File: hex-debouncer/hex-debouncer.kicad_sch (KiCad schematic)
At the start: 37 parts, among them J1 Conn_01x08, SW1 A, SW2 B, SW3 C, SW4 D, SW5 E, SW6 F, U1 74HC14

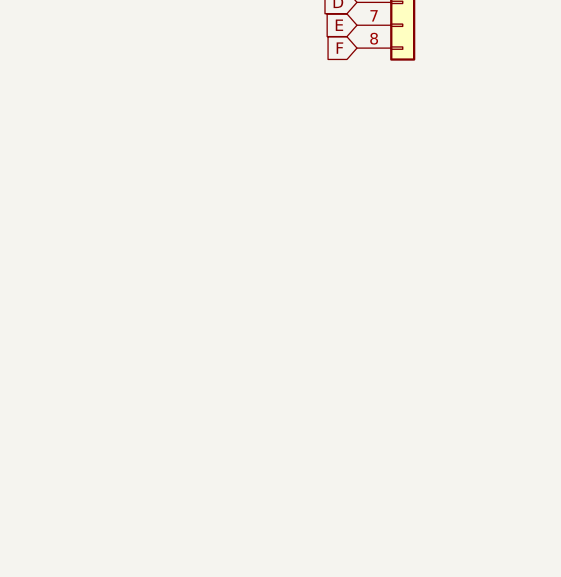
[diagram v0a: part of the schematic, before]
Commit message: up
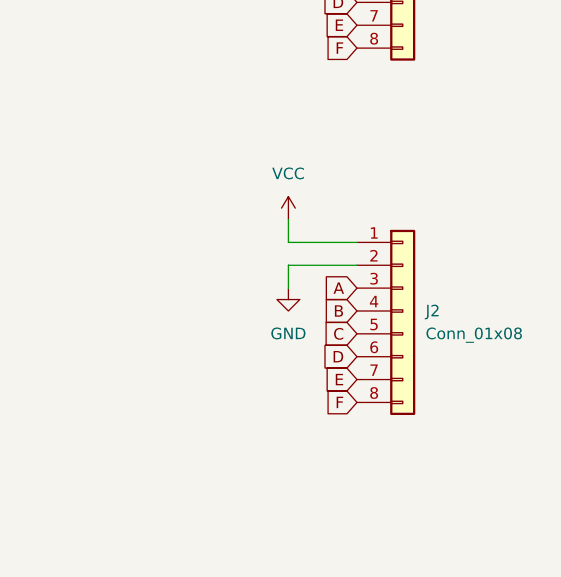
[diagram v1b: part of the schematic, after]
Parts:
- added J2: Conn_01x08, Connector_PinHeader_2.54mm:PinHeader_1x08_P2.54mm_Vertical, symbol Connector_Generic:Conn_01x08
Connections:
- net A: now also J2.3 (Pin_3)
- net B: now also J2.4 (Pin_4)
- net C: now also J2.5 (Pin_5)
- net D: now also J2.6 (Pin_6)
- net E: now also J2.7 (Pin_7)
- net F: now also J2.8 (Pin_8)
- net GND: now also J2.2 (Pin_2)
- net VCC: now also J2.1 (Pin_1)
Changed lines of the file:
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@@
+    (stroke (width 0) (type default) (color 0 0 0 0))
+  )
+  (wire (pts (xy 246.38 81.28) (xy 246.38 83.82))
     (stroke (width 0) (type default) (color 0 0 0 0))
   )
@@
     (stroke (width 0) (type default) (color 0 0 0 0))
   )
+  (wire (pts (xy 254 81.28) (xy 246.38 81.28))
+    (stroke (width 0) (type default) (color 0 0 0 0))
+  )
   (wire (pts (xy 107.95 43.18) (xy 107.95 45.72))
     (stroke (width 0) (type default) (color 0 0 0 0))
@@
     (stroke (width 0) (type default) (color 0 0 0 0))
   )
+  (wire (pts (xy 254 78.74) (xy 246.38 78.74))
+    (stroke (width 0) (type default) (color 0 0 0 0))
+  )
   (wire (pts (xy 64.77 43.18) (xy 64.77 45.72))
     (stroke (width 0) (type default) (color 0 0 0 0))
@@
   )
   (wire (pts (xy 123.19 38.1) (xy 123.19 43.18))
+    (stroke (width 0) (type default) (color 0 0 0 0))
+  )
+  (wire (pts (xy 246.38 76.2) (xy 246.38 78.74))
     (stroke (width 0) (type default) (color 0 0 0 0))
   )
@@
     )
   )
+  (global_label "D" (shape input) (at 254 91.44 180) (fields_autoplaced)
+    (effects (font (size 1.27 1.27)) (justify right))
+    (property "Intersheet References" "${INTERSHEET_REFS}" (id 0) (at 250.3169 91.5194 0)
+      (effects (font (size 1.27 1.27)) (justify right) hide)
+    )
+  )
   (global_label "D" (shape input) (at 254 52.07 180) (fields_autoplaced)
     (effects (font (size 1.27 1.27)) (justify right))
@@
     )
   )
+  (global_label "A" (shape input) (at 254 83.82 180) (fields_autoplaced)
+    (effects (font (size 1.27 1.27)) (justify right))
+    (property "Intersheet References" "${INTERSHEET_REFS}" (id 0) (at 250.4983 83.8994 0)
+      (effects (font (size 1.27 1.27)) (justify right) hide)
+    )
+  )
   (global_label "D" (shape input) (at 97.79 86.36 0) (fields_autoplaced)
     (effects (font (size 1.27 1.27)) (justify left))
@@
     )
   )
+  (global_label "C" (shape input) (at 254 88.9 180) (fields_autoplaced)
+    (effects (font (size 1.27 1.27)) (justify right))
+    (property "Intersheet References" "${INTERSHEET_REFS}" (id 0) (at 250.3169 88.9794 0)
+      (effects (font (size 1.27 1.27)) (justify right) hide)
+    )
+  )
   (global_label "F" (shape input) (at 254 57.15 180) (fields_autoplaced)
     (effects (font (size 1.27 1.27)) (justify right))
@@
     )
   )
+  (global_label "E" (shape input) (at 254 93.98 180) (fields_autoplaced)
+    (effects (font (size 1.27 1.27)) (justify right))
+    (property "Intersheet References" "${INTERSHEET_REFS}" (id 0) (at 250.4379 94.0594 0)
+      (effects (font (size 1.27 1.27)) (justify right) hide)
+    )
+  )
   (global_label "F" (shape input) (at 140.97 86.36 0) (fields_autoplaced)
     (effects (font (size 1.27 1.27)) (justify left))
     (property "Intersheet References" "${INTERSHEET_REFS}" (id 0) (at 144.4717 86.2806 0)
       (effects (font (size 1.27 1.27)) (justify left) hide)
+    )
+  )
+  (global_label "B" (shape input) (at 254 86.36 180) (fields_autoplaced)
+    (effects (font (size 1.27 1.27)) (justify right))
+    (property "Intersheet References" "${INTERSHEET_REFS}" (id 0) (at 250.3169 86.4394 0)
+      (effects (font (size 1.27 1.27)) (justify right) hide)
+    )
+  )
+  (global_label "F" (shape input) (at 254 96.52 180) (fields_autoplaced)
+    (effects (font (size 1.27 1.27)) (justify right))
+    (property "Intersheet References" "${INTERSHEET_REFS}" (id 0) (at 250.4983 96.5994 0)
+      (effects (font (size 1.27 1.27)) (justify right) hide)
     )
   )
@@
     (pin "7")
   )
+  (symbol (lib_id "power:VCC") (at 246.38 76.2 0) (unit 1)
+    (in_bom yes) (on_board yes) (fields_autoplaced)
+    (property "Reference" "#PWR028" (id 0) (at 246.38 80.01 0)
+      (effects (font (size 1.27 1.27)) hide)
+    )
+    (property "Value" "VCC" (id 1) (at 246.38 71.12 0))
+    (property "Footprint" "" (id 2) (at 246.38 76.2 0)
+      (effects (font (size 1.27 1.27)) hide)
+    )
+    (property "Datasheet" "" (id 3) (at 246.38 76.2 0)
+      (effects (font (size 1.27 1.27)) hide)
+    )
+    (pin "1")
+  )
   (symbol (lib_id "Diode:LL4148") (at 30.48 86.36 180) (unit 1)
     (in_bom yes) (on_board yes) (fields_autoplaced)
@@
     (pin "1")
     (pin "2")
+  )
+  (symbol (lib_id "power:GND") (at 246.38 83.82 0) (unit 1)
+    (in_bom yes) (on_board yes)
+    (property "Reference" "#PWR029" (id 0) (at 246.38 90.17 0)
+      (effects (font (size 1.27 1.27)) hide)
+    )
+    (property "Value" "GND" (id 1) (at 246.38 88.9 0))
+    (property "Footprint" "" (id 2) (at 246.38 83.82 0)
+      (effects (font (size 1.27 1.27)) hide)
+    )
+    (property "Datasheet" "" (id 3) (at 246.38 83.82 0)
+      (effects (font (size 1.27 1.27)) hide)
+    )
+    (pin "1")
   )
   (symbol (lib_id "74xx:74HC14") (at 46.99 86.36 0) (unit 2)
@@
     (pin "1")
   )
+  (symbol (lib_id "Connector_Generic:Conn_01x08") (at 259.08 86.36 0) (unit 1)
+    (in_bom yes) (on_board yes) (fields_autoplaced)
+    (property "Reference" "J2" (id 0) (at 261.62 86.3599 0)
+      (effects (font (size 1.27 1.27)) (justify left))
+    )
+    (property "Value" "Conn_01x08" (id 1) (at 261.62 88.8999 0)
+      (effects (font (size 1.27 1.27)) (justify left))
+    )
+    (property "Footprint" "Connector_PinHeader_2.54mm:PinHeader_1x08_P2.54mm_Vertical" (id 2) (at 259.08 86.36 0)
+      (effects (font (size 1.27 1.27)) hide)
+    )
+    (property "Datasheet" "~" (id 3) (at 259.08 86.36 0)
+      (effects (font (size 1.27 1.27)) hide)
+    )
+    (pin "1")
+    (pin "2")
+    (pin "3")
+    (pin "4")
+    (pin "5")
+    (pin "6")
+    (pin "7")
+    (pin "8")
+  )
   (symbol (lib_id "Device:C") (at 123.19 52.07 0) (unit 1)
     (in_bom yes) (on_board yes) (fields_autoplaced)
@@
       (reference "#PWR027") (unit 1) (value "GND") (footprint "")
     )
+    (path "/2bfebc01-56e4-4ab9-8a66-4e2193c9c3d5"
+      (reference "#PWR028") (unit 1) (value "VCC") (footprint "")
+    )
+    (path "/539257a9-0e86-4e3c-9d9c-4c6a64c499d8"
+      (reference "#PWR029") (unit 1) (value "GND") (footprint "")
+    )
     (path "/f08a42c6-aa17-41ee-ae4f-8bb291ce2f52"
       (reference "C1") (unit 1) (value "100nF") (footprint "Capacitor_SMD:C_0805_2012Metric")
@@
       (reference "J1") (unit 1) (value "Conn_01x08") (footprint "Connector_PinHeader_2.54mm:PinHeader_1x08_P2.54mm_Vertical")
     )
+    (path "/e0a605fc-c78f-4097-a89a-bf7f8109a7a4"
+      (reference "J2") (unit 1) (value "Conn_01x08") (footprint "Connector_PinHeader_2.54mm:PinHeader_1x08_P2.54mm_Vertical")
+    )
     (path "/bcb299c0-3d24-4466-a101-3cc4d39009f6"
